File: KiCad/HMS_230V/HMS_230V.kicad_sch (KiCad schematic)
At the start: 11 parts, among them SW1 SWITCH_1, SW2 SWITCH_2, U1 Circulator_Gas, U2 Circulator_Wood, U3 Pipe_Thermostat_Gas, U4 Pipe_Thermostat_Wood, U5 Ball_Valve_Gas, U6 Ball_Valve_Wood, U8 MVPDM-1PHS, U9 MVPDM-1PHS

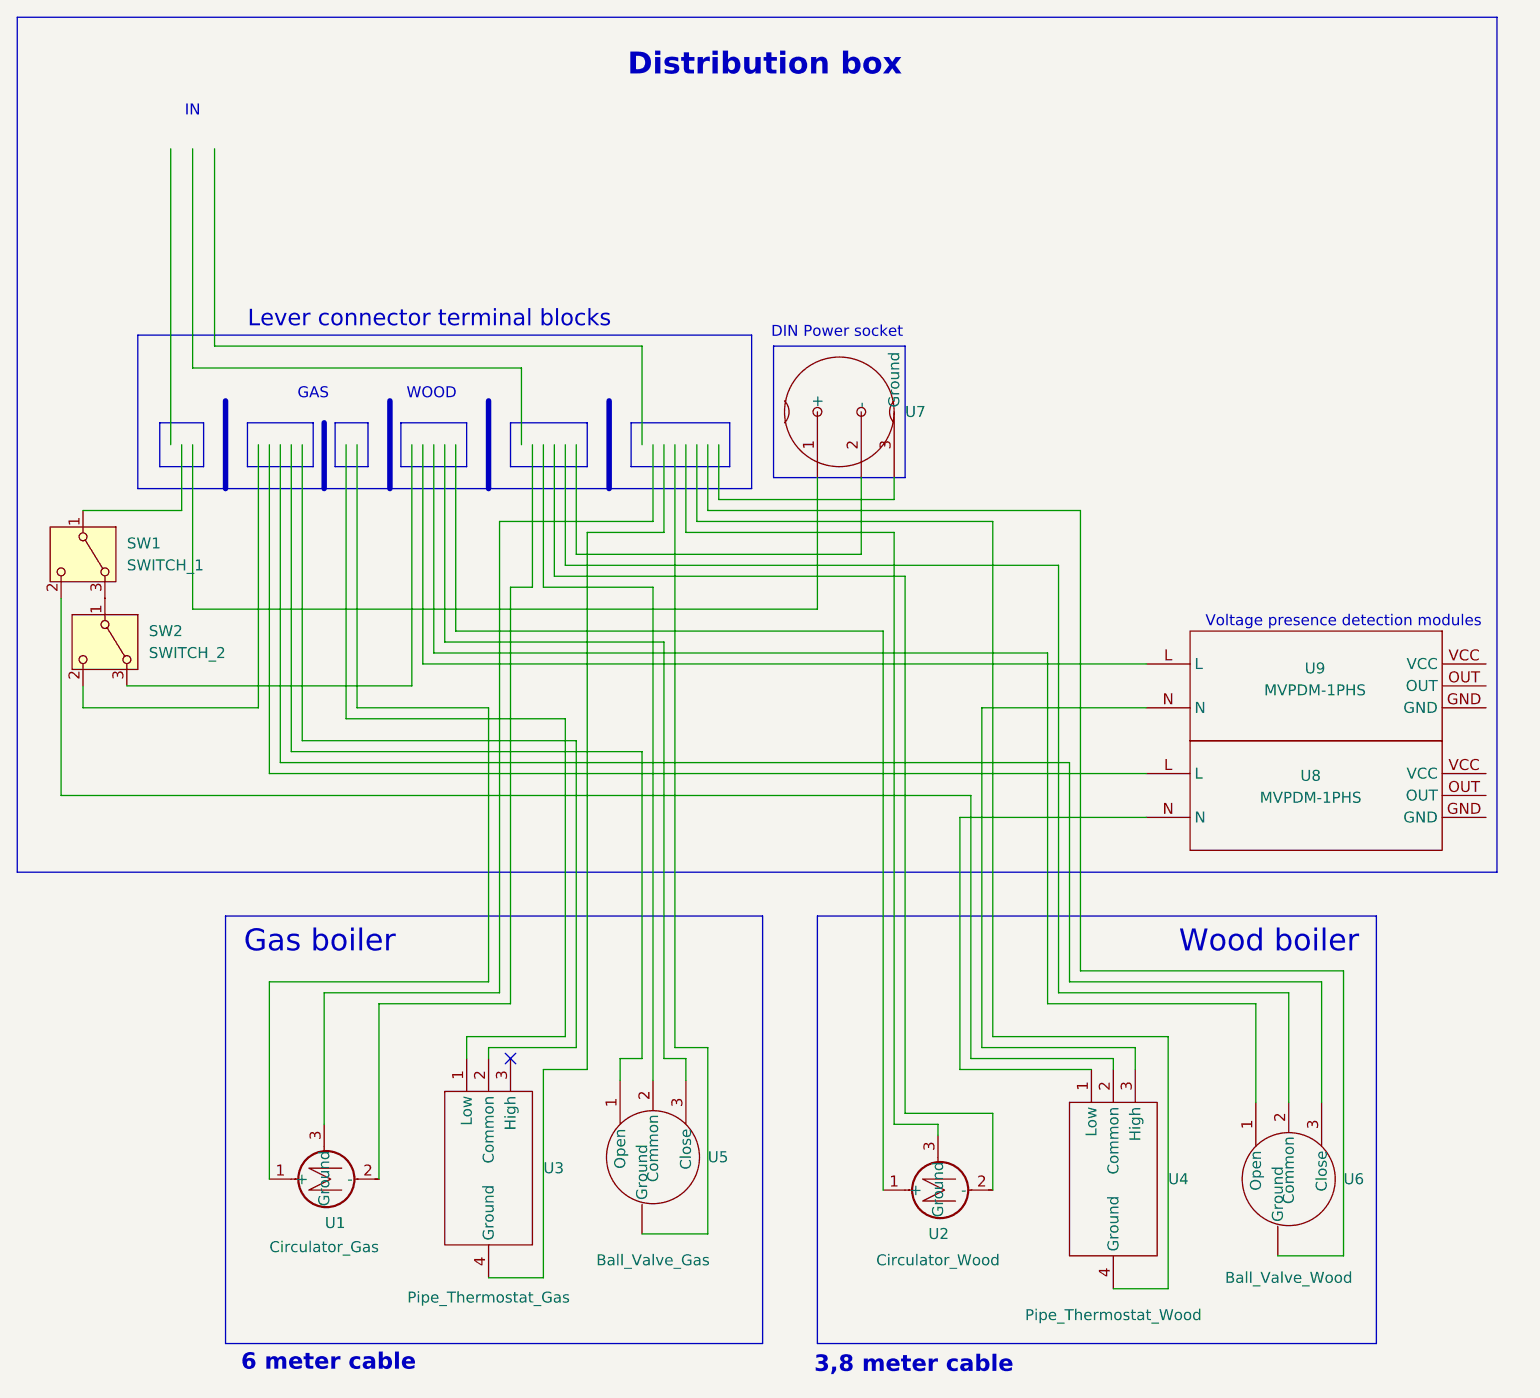
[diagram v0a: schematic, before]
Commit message: Sensor manager and data manager finalization
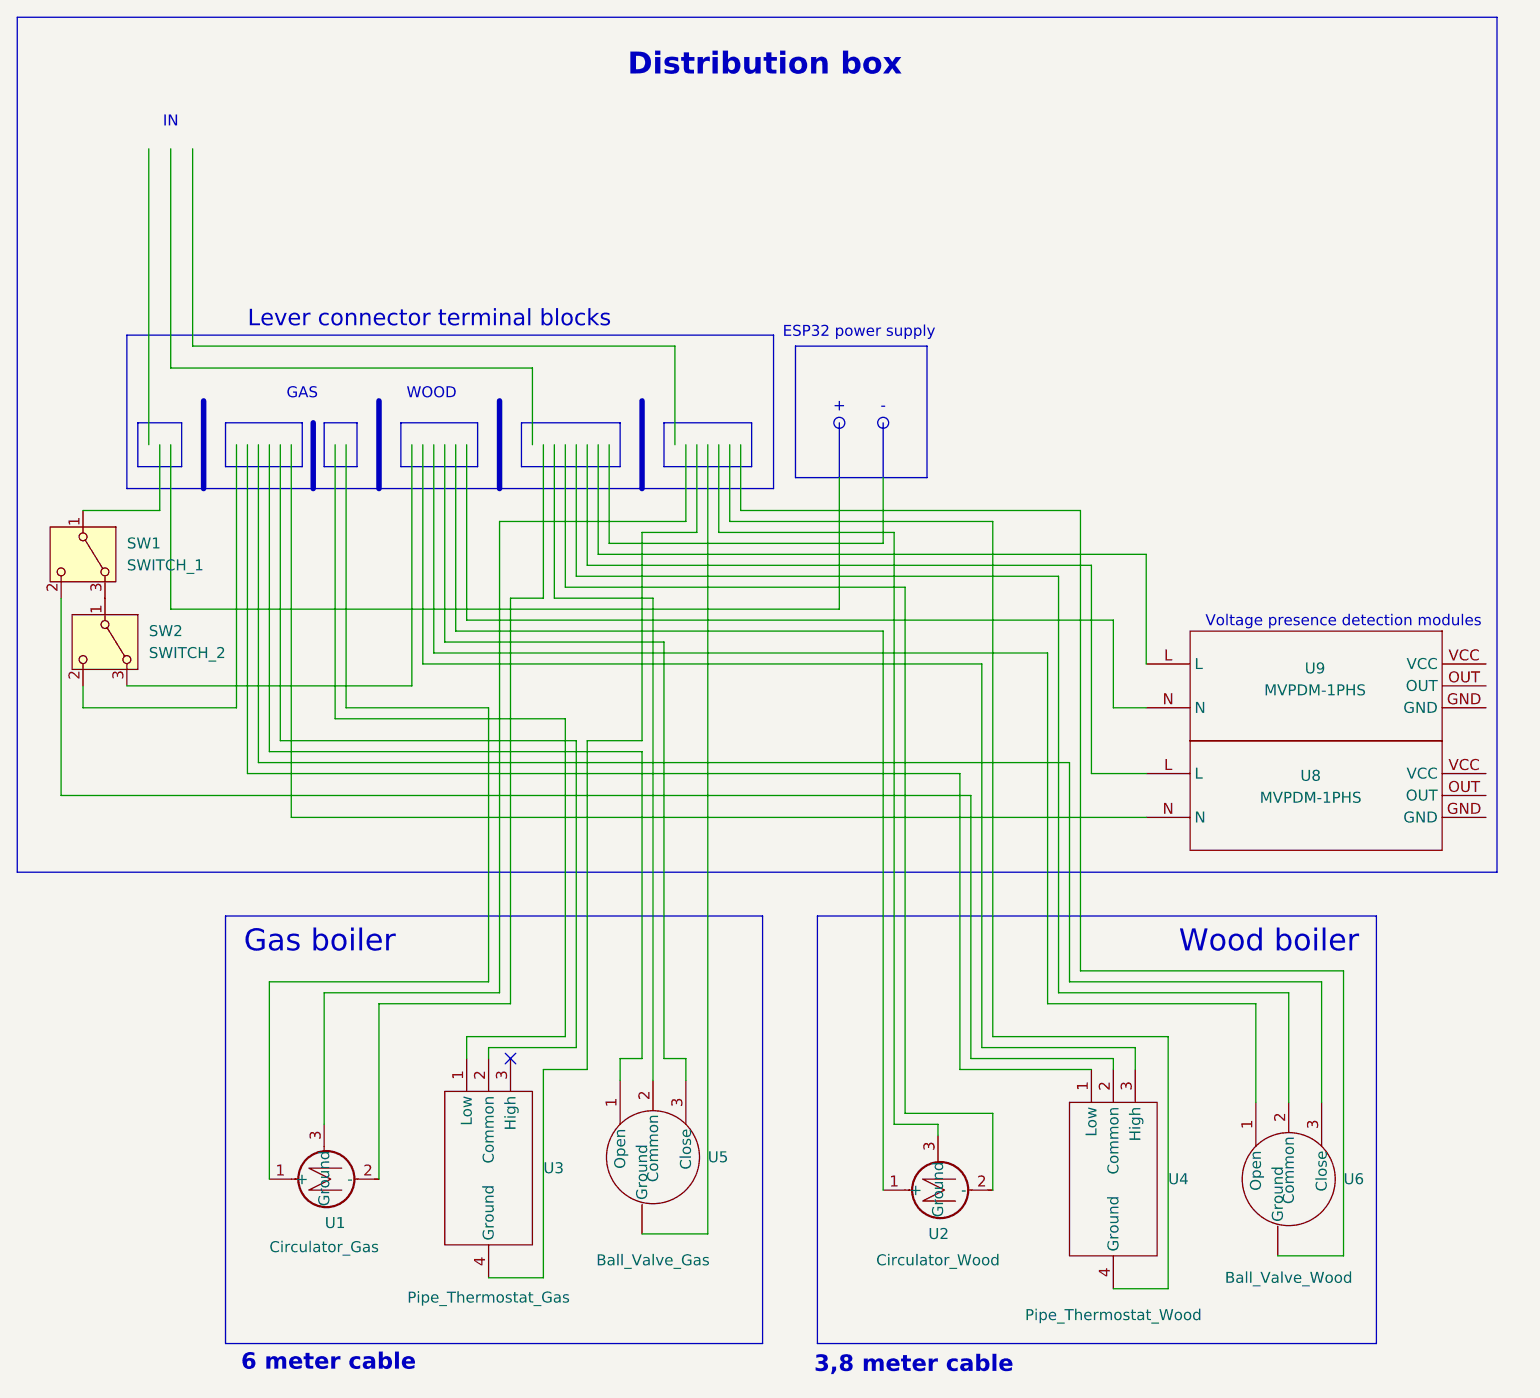
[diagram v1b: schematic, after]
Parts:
- removed U7: (no value), symbol HMS_Symbols:Connector_Grounded
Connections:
- net at U4.1 (Low): no longer U8.N
- net at U4.3 (High): no longer U9.N
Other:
- note added: "+"
- note added: "-"
- note added: "ESP32 power supply"
- note removed: "DIN Power socket"
